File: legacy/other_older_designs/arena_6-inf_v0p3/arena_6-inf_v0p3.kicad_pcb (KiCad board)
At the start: 2 copper layers, 260 x 60 mm, 39 parts, among them M1 VAL**, M2 VAL**, M3 VAL**, M4 VAL**, M5 VAL**, M6 VAL**, P1 CONN15, P10 CONN_20X2, P2 CONN15, P3 CONN15, P4 CONN15, P5 CONN15, P6 CONN15, P7 CONN_20X2, P8 CONN_34X2, P9 CONN_2, Q1 MOSFET_NCHAN, SW1 SWITCH_INV, U1 SPARKFUN_TXB0104, U2 SPARKFUN_TXB0104, U3 SPARKFUN_TXB0104, U4 SPARKFUN_TXB0104, U5 SPARKFUN_TXB0104, U6 SPARKFUN_TXB0104, U7 SPARKFUN_TXB0104, U8 POLOLU_3V3

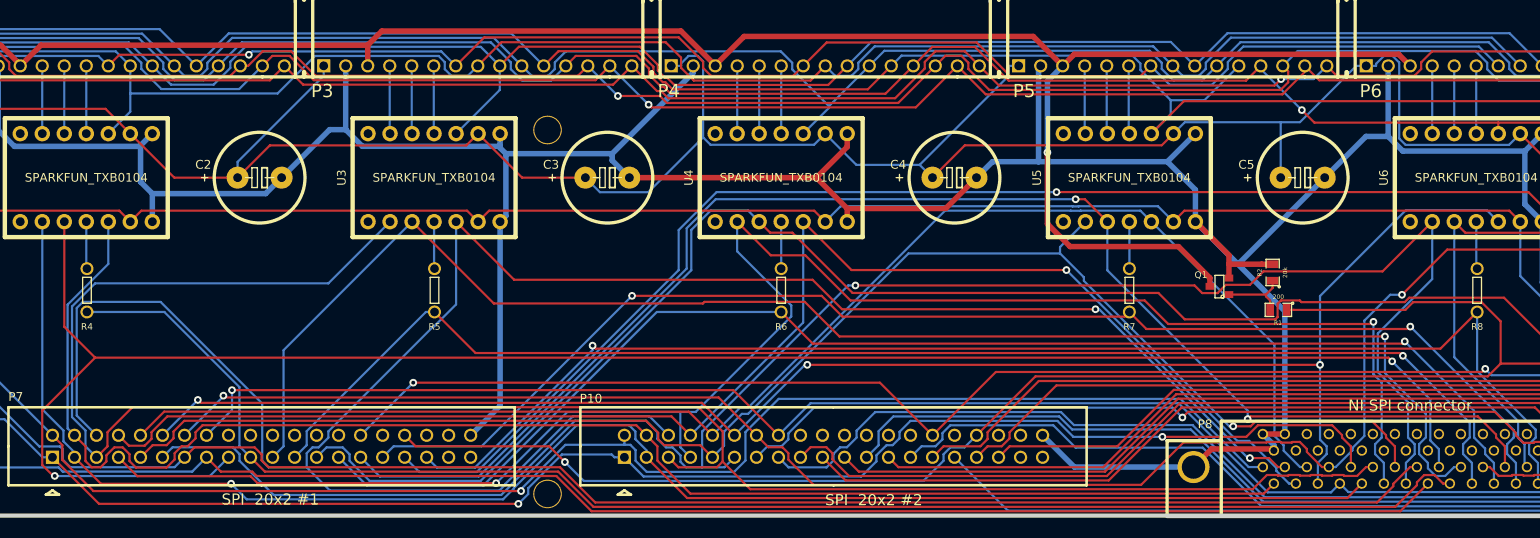
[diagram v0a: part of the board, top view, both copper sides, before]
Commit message: Intermediate save during re-route of NI 12-12 arena with vreg.
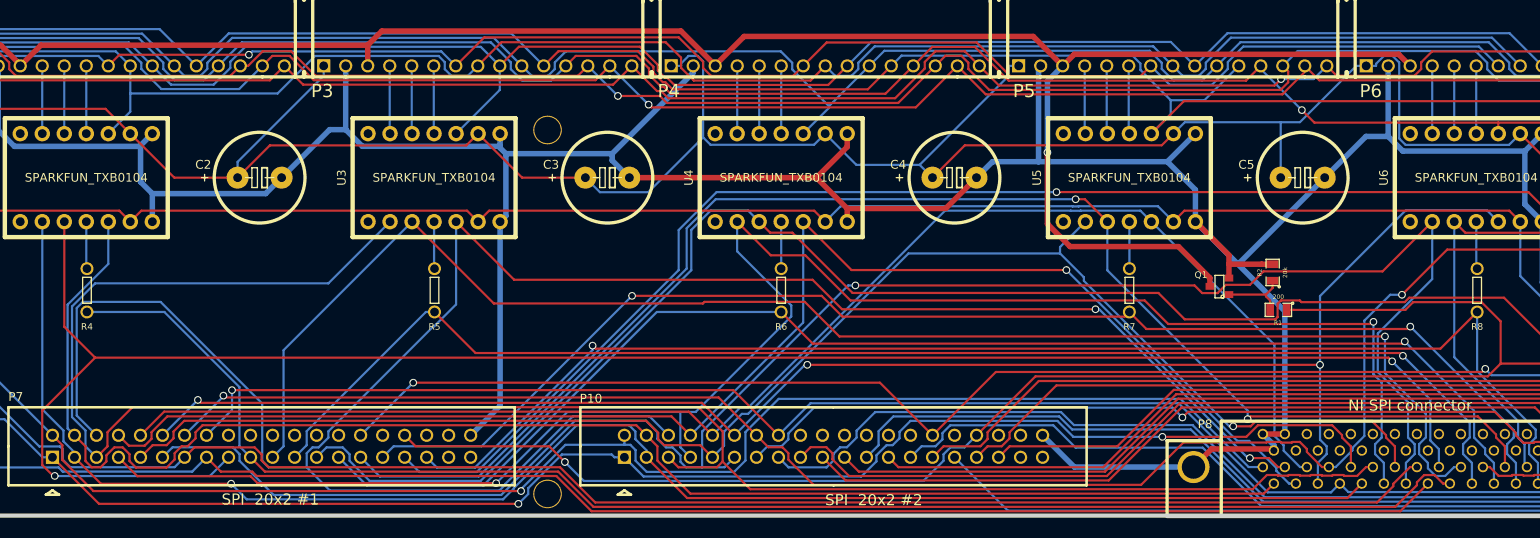
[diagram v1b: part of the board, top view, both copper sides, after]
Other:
- net class Default removed
- net class Pwr removed
- net class Reset_Pan removed
